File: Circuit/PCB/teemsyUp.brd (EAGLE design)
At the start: 71.1 x 145.7 mm, 34 parts

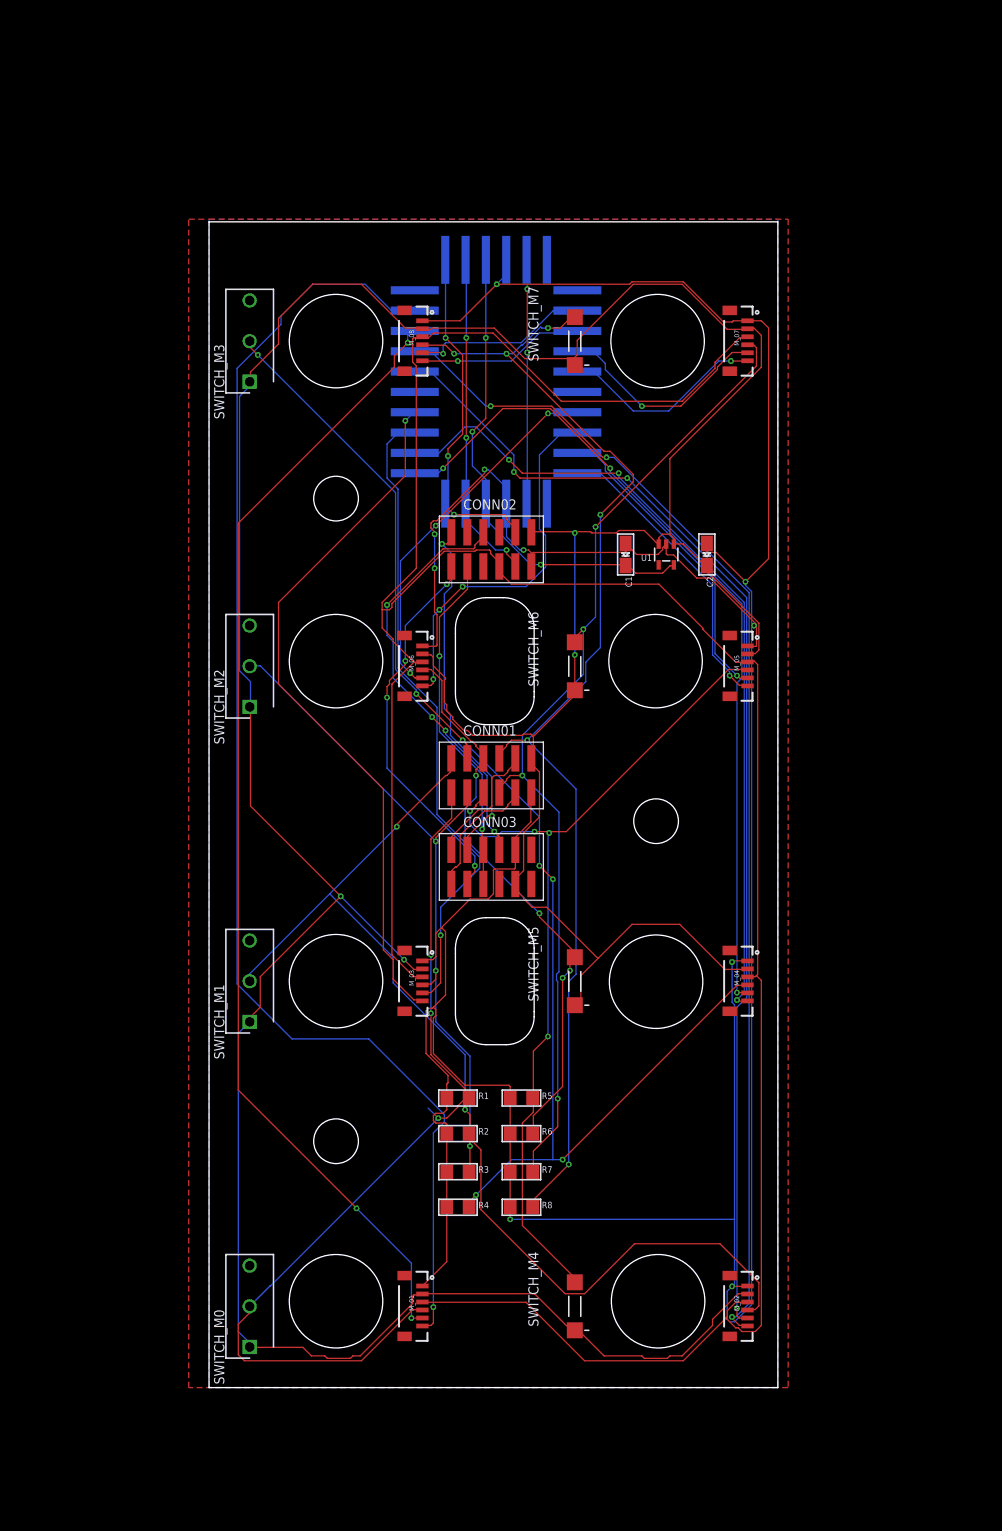
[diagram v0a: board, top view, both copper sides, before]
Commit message: PCB
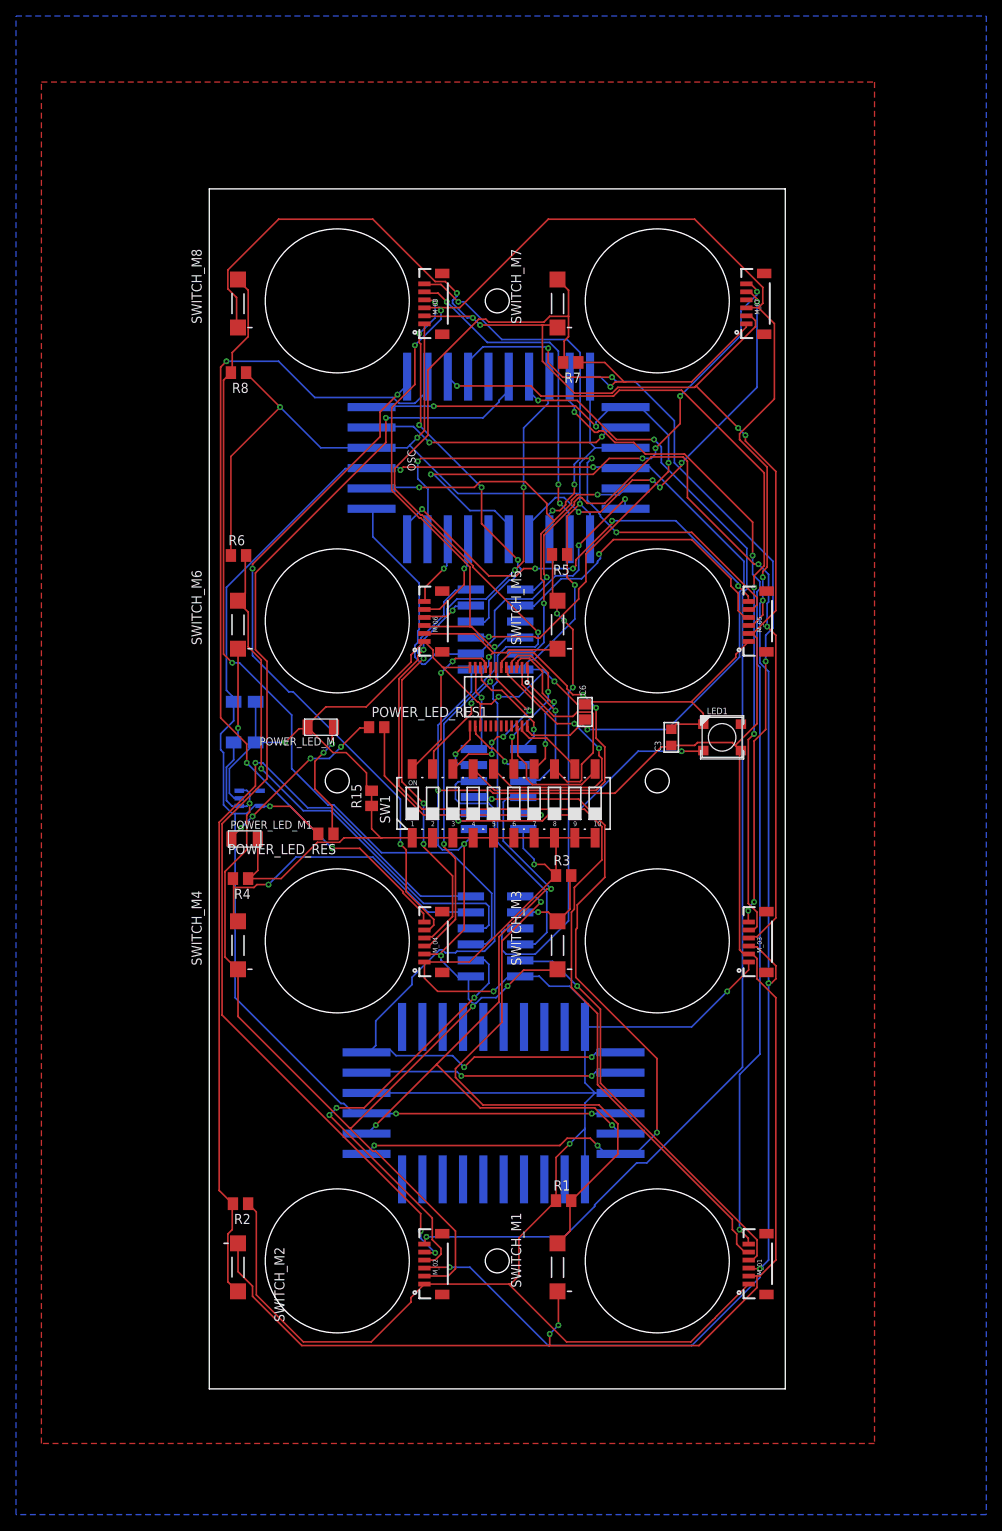
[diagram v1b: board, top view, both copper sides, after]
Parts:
- removed SWITCH_M0: D2F-5, D2F-5:SHDR3W100P0X508_1X3_1280X580X5
- added C3: 0.1uf, rc-master-smd:C0805
- added C6: 0.1uf, microbuilder:0805
- added J5, J6, J7, J8: (no value), SparkFun-Connectors:1X10_SMD_MALE
- added LED1: (no value), SK6812:LED5050_N
- added POWER_LED_M, POWER_LED_M1: LEDFAB1206, fab:LED1206FAB
- added POWER_LED_RES: 500, resistor:M0805
- added POWER_LED_RES1: 500, resistor:R0805
- added R15: (no value), resistor:M0805
- added SW1: 219-10, switch-dil:CTS-219-10
- added SWITCH_M8: DTSM-3, switch-tact:DTSM-3
- added U3: MUX-74HC4067, SparkFun:SSOP24
- J3, J4: device SparkFun-Connectors:1X10_SMD_MALE -> SparkFun-Connectors:1X06_SMD_MALE
- R1, R2, R3, R5, R6, R7, R8: value (none) -> 10k; device microbuilder:1206 -> resistor:M0805
- R4: value (none) -> 10K; device microbuilder:1206 -> resistor:M0805
- SWITCH_M1, SWITCH_M2, SWITCH_M3: value D2F-5 -> DTSM-3; device D2F-5:SHDR3W100P0X508_1X3_1280X580X5 -> switch-tact:DTSM-3
- moved R8 110.2 mm to (3.68, 126.9), turned to 180 degrees
- moved R7 101.3 mm to (45.2, 128.1), turned to 180 degrees
- moved R6 80.5 mm to (3.68, 104.0)
- moved SWITCH_M3 80.3 mm to (43.6, 55.3)
- moved J3 72.6 mm to (19.7, 41.9), turned to 270 degrees
- moved J4 72.6 mm to (51.4, 41.9), turned to 270 degrees
- moved SWITCH_M2 70.1 mm to (3.62, 15.0), turned to 270 degrees
- moved R5 68.1 mm to (43.8, 104.1), turned to 180 degrees
- moved C2 62.4 mm to (4.45, 80.6), flipped to the bottom, turned to 0 degrees
- moved SWITCH_M4 61.7 mm to (3.62, 55.3)
- moved U1 60.3 mm to (5.08, 73.7), flipped to the bottom, turned to 90 degrees
- moved C1 51.1 mm to (4.45, 85.7), flipped to the bottom, turned to 0 degrees
- moved R4 49.3 mm to (3.94, 63.6), turned to 180 degrees
- moved SWITCH_M1 49.2 mm to (43.6, 15.0)
- moved SWITCH_M5 44.6 mm to (43.6, 95.4)
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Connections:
- net MUX_RESET renamed !RESET_SX0
- net S_SCL renamed SCL_SX0
- net S_SDA renamed SDA_SX0
- removed net I2CS_0: J3.9, M_01.6
- removed net I2CS_1: J3.8, M_01.5
- removed net I2CS_10: J4.3, M_06.6
- removed net I2CS_11: J4.4, M_06.5
- removed net I2CS_12: J4.6, M_07.6
- removed net I2CS_13: J4.7, M_07.5
- removed net I2CS_14: J4.8, M_08.6
- removed net I2CS_15: J4.9, M_08.5
- removed net I2CS_2: J3.7, M_02.6
- removed net I2CS_3: J3.6, M_02.5
- removed net I2CS_4: J3.4, M_03.6
- removed net I2CS_5: J3.3, M_03.5
- removed net I2CS_6: J3.2, M_04.6
- removed net I2CS_7: J3.1, M_04.5
- removed net I2CS_8: J4.1, M_05.6
- removed net I2CS_9: J4.2, M_05.5
- removed net MUX_INT: J1.1
- removed net MUX_OSCIO: J2.1
- removed net N$16: SWITCH_M3.3
- removed net N$19: SWITCH_M0.3
- removed net N$22: CONN03.12
- removed net S_SEN_01: CONN02.8
- removed net VCC1: J3.5
- removed net VCC2: J4.5
- new net !INT_SX0: CONN02.8, J1.1, J2.1
- new net !INT_SX1: CONN03.6, J3.1, J4.1
- new net !RESET_SX1: J3.2, J4.2
- new net 0_SX0: J5.2, M_01.6
- new net 0_SX1: J7.2
- new net 10_SX0: J6.3, M_06.6
- new net 10_SX1: J8.3
- new net 11_SX0: J6.4, M_06.5
- new net 11_SX1: J8.4
- new net 12_SX0: J6.6, M_07.6
- new net 12_SX1: J8.6
- new net 13_SX0: J6.7, M_07.5
- new net 13_SX1: J8.7
- new net 14_SX0: J6.8, M_08.6
- new net 14_SX1: J8.8
- new net 15_SX0: J6.9, M_08.5
- new net 15_SX1: J8.9
- new net 1_SX0: J5.3, M_01.5
- new net 1_SX1: J7.3
- new net 2_SX0: J5.4, M_02.6
- new net 2_SX1: J7.4
- new net 3_SX0: J5.5, M_02.5
- new net 3_SX1: J7.5
- new net 4_SX0: J5.7, M_03.6
- new net 4_SX1: J7.7
- new net 5_SX0: J5.8, M_03.5
- new net 5_SX1: J7.8
- new net 6_SX0: J5.9, M_04.6
- new net 6_SX1: J7.9
- new net 7_SX0: J5.10, M_04.5
- new net 7_SX1: J7.10
- new net 8_SX0: J6.1, M_05.6
- new net 8_SX1: J8.1
- new net 9_SX0: J6.2, M_05.5
- new net 9_SX1: J8.2
- new net C0: SW1.20, U3.9
- new net C1: SW1.19, U3.8
- new net C2: SW1.18, U3.7
- new net C3: SW1.17, U3.6
- new net C4: SW1.16, U3.5
- new net C5: SW1.15, U3.4
- new net C6: SW1.14, U3.3
- new net C7: SW1.13, U3.2
- new net C8: SW1.12, U3.23
- new net C9: SW1.11, U3.22
- new net LED_DEBUG: CONN03.10, LED1.4-DIN
- new net LED_ST: CONN03.9, POWER_LED_RES1.2
- new net MUX_S0: CONN03.1, U3.10
- new net MUX_S1: CONN03.2, U3.11
- new net MUX_S2: CONN03.3, U3.14
- new net MUX_S3: CONN03.4, U3.13
- new net MUX_SIG: CONN03.5, U3.1
- new net N$1: POWER_LED_M1.1, POWER_LED_RES1.1
- new net N$11: POWER_LED_M.1, POWER_LED_RES.1
- new net N$13: LED1.2-DOUT
- new net N$29: J8.5
- new net SCL_SX1: CONN03.8, J3.6, J4.6
- new net SDA_SX1: CONN03.7, J3.5, J4.5
- net 3.3V: now also C6.1, J3.4, J4.4, POWER_LED_RES.2, U3.24
- net GND_MCU: now also C3.2, C6.2, CONN03.12, J3.3, J4.3, J5.1, J6.10, J7.1, J8.10, LED1.3-GND, POWER_LED_M.2, POWER_LED_M1.2, R15.1, R15.2, SW1.1, SW1.10, SW1.2, SW1.3, SW1.4, SW1.5, SW1.6, SW1.7, SW1.8, SW1.9, U3.12, U3.15; no longer CONN03.10
- net I2CM_0: now also SWITCH_M1.2; no longer M_01.4, SWITCH_M0.2
- net I2CM_1: now also SWITCH_M2.2; no longer M_02.4, SWITCH_M1.2
- net I2CM_10: now also M_03.4; no longer CONN03.3
- net I2CM_11: now also M_04.4; no longer CONN03.4
- net I2CM_12: now also M_05.4; no longer CONN03.5, CONN03.6
- net I2CM_13: now also M_06.4
- net I2CM_14: now also M_07.4; no longer CONN03.7
- net I2CM_15: now also M_08.4; no longer CONN03.8
- net I2CM_2: now also SWITCH_M3.2; no longer M_03.4, SWITCH_M2.2
- net I2CM_3: now also SWITCH_M4.2; no longer M_04.4, SWITCH_M3.2
- net I2CM_4: now also SWITCH_M5.2; no longer M_05.4, SWITCH_M4.2
- net I2CM_5: now also SWITCH_M6.2; no longer M_06.4, SWITCH_M5.2
- net I2CM_6: now also SWITCH_M7.2; no longer M_07.4, SWITCH_M6.2
- net I2CM_7: now also SWITCH_M8.2; no longer M_08.4, SWITCH_M7.2
- net I2CM_8: now also M_01.4; no longer CONN03.1
- net I2CM_9: now also M_02.4; no longer CONN03.2
- net N$12: now also J5.6; no longer CONN03.11
- net N$17: now also J7.6; no longer SWITCH_M2.3
- net N$18: now also J6.5; no longer SWITCH_M1.3
- net VCC_MCU: now also C3.1, CONN03.11, LED1.1-VDD, SWITCH_M8.1; no longer CONN03.9, SWITCH_M0.1
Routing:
- net 3.3V: track 60.7 -> 241.6 mm, vias 3 -> 6
- net I2CS_0: track 166.4 -> 0.00 mm, vias 1 -> 0
- net 2_SX0: track 0.00 -> 152.9 mm, vias 0 -> 3
- net 1_SX0: track 0.00 -> 152.8 mm, vias 0 -> 3
- net I2CS_2: track 148.5 -> 0.00 mm, vias 3 -> 0
- net I2CS_3: track 146.2 -> 0.00 mm, vias 3 -> 0
- net 3_SX0: track 0.00 -> 145.1 mm, vias 0 -> 3
- net I2CS_1: track 143.1 -> 0.00 mm, vias 3 -> 0
- net GND_MCU: track 463.4 -> 592.6 mm, vias 10 -> 12
- net I2CM_3: track 167.3 -> 39.8 mm, vias 7 -> 1
- net 0_SX0: track 0.00 -> 125.4 mm, vias 0 -> 3
- net 6_SX0: track 0.00 -> 112.7 mm, vias 0 -> 3
- net I2CS_7: track 104.8 -> 0.00 mm, vias 3 -> 0
- net 5_SX0: track 0.00 -> 104.3 mm, vias 0 -> 3
- net I2CS_6: track 103.5 -> 0.00 mm, vias 3 -> 0
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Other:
- board size 71.1 x 145.7 mm -> 72 x 150 mm
- board text added: "!RST"
- board text added: "3.3V"
- board text added: "GND"
- board text added: "OSC"
- board text added: "SCL"
- board text added: "SDA"
